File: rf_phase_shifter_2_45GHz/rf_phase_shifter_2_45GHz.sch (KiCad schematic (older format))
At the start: 12 parts, among them J1 CON-SMA-EDGE-S, J2 CON-SMA-EDGE-S, J3 CON-SMA-EDGE-S

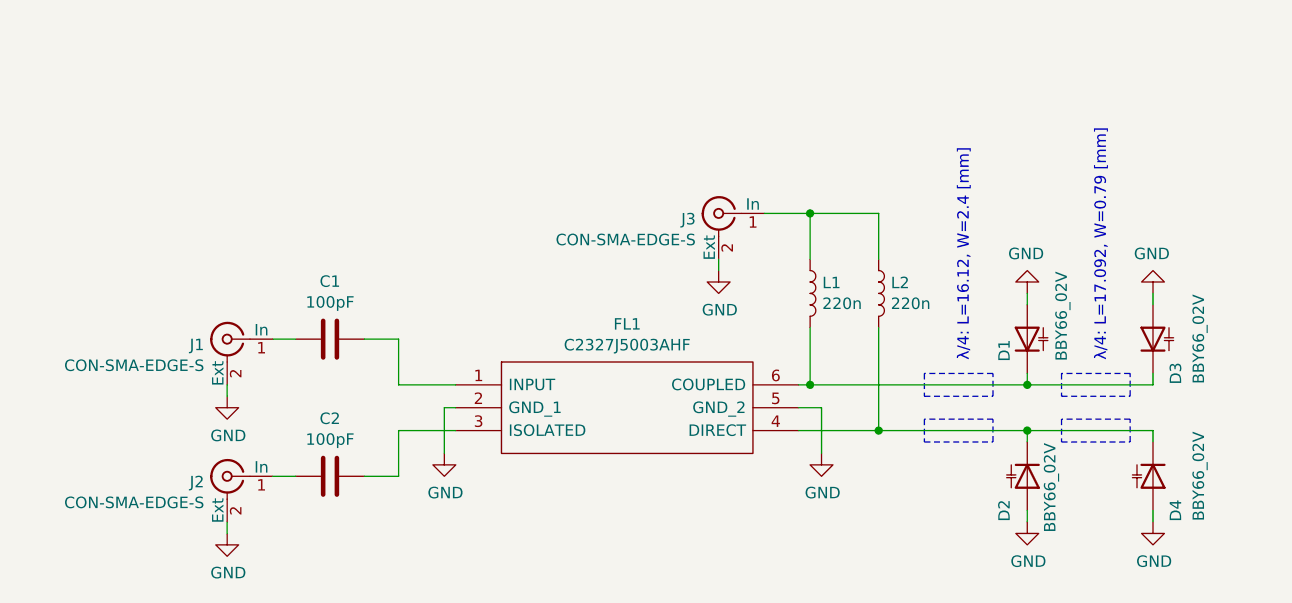
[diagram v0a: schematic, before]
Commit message: finished pcb layouts
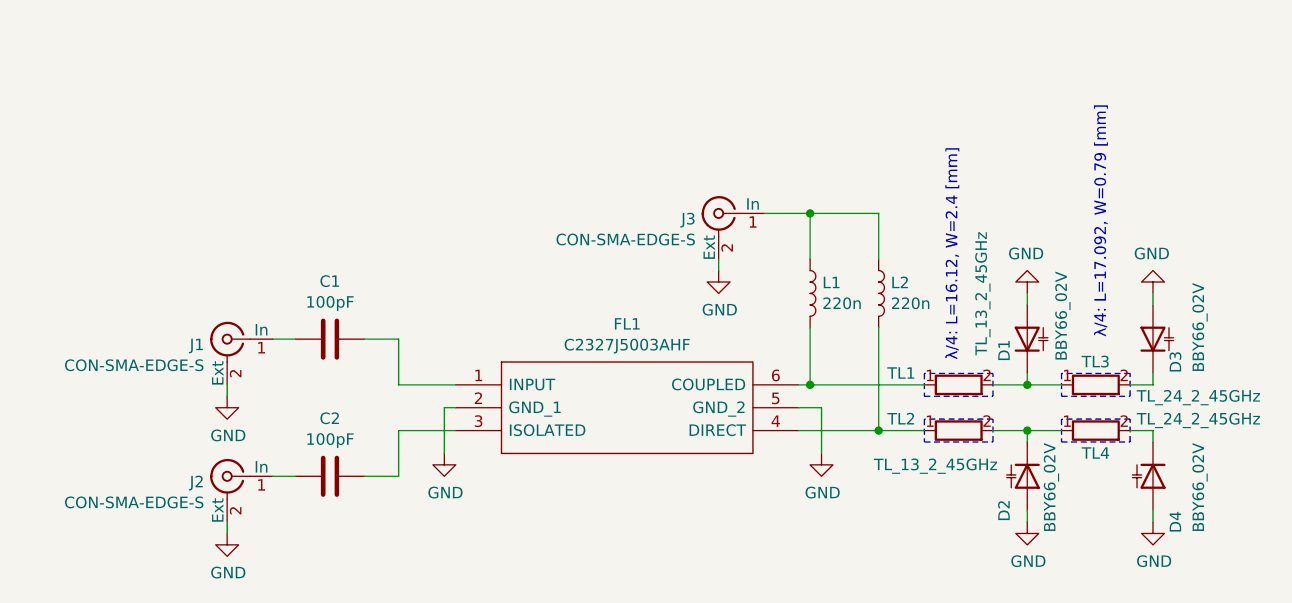
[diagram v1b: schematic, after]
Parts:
- added TL1, TL2: TL_13_2_45GHz, analog_rf_phase_shifter_module:TL_13_2_45GHz, symbol analog_rf_phase_shifter_module:TL_13_2_45GHz
- added TL3, TL4: TL_24_2_45GHz, analog_rf_phase_shifter_module:TL_24_2_45GHz, symbol analog_rf_phase_shifter_module:TL_24_2_45GHz
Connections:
- net at FL1.6 (COUPLED), L1.2: now also TL1.1; no longer D1.1 (K), D3.1 (K)
- net at FL1.4 (DIRECT), L2.2: now also TL2.1; no longer D2.1 (K), D4.1 (K)
- new net: D1.1 (K), TL1.2, TL3.1
- new net: D2.1 (K), TL2.2, TL4.1
- new net: D3.1 (K), TL3.2
- new net: D4.1 (K), TL4.2
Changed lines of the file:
@@
 U 1 1 60376509
 P 5600 2550
-F 0 "D4" H 5750 2650 50  0000 C CNN
-F 1 "BBY66_02V" H 5600 2750 50  0000 C CNN
+F 0 "D4" H 5800 2650 50  0000 C CNN
+F 1 "BBY66_02V" H 5650 2750 50  0000 C CNN
 F 2 "Diode_SMD:D_SOD-523" H 5600 2550 50  0001 C CNN
 F 3 "~" H 5600 2550 50  0001 C CNN
@@
 U 1 1 60375EF1
 P 5600 1950
-F 0 "D3" H 5450 1850 50  0000 C CNN
-F 1 "BBY66_02V" H 5600 1750 50  0000 C CNN
+F 0 "D3" H 5500 1850 50  0000 C CNN
+F 1 "BBY66_02V" H 5650 1750 50  0000 C CNN
 F 2 "Diode_SMD:D_SOD-523" H 5600 1950 50  0001 C CNN
 F 3 "~" H 5600 1950 50  0001 C CNN
@@
 $EndComp
 Wire Wire Line
-	5050 2150 5600 2150
-Wire Wire Line
-	5050 2350 5600 2350
-Wire Wire Line
-	4400 2350 5050 2350
+	5050 2150 5200 2150
+Wire Wire Line
+	5050 2350 5200 2350
+Wire Wire Line
+	4400 2350 4600 2350
 Connection ~ 5050 2150
 Connection ~ 4100 2150
 Wire Wire Line
-	4100 2150 5050 2150
-Text Notes 4800 2050 1    50   ~ 0
+	4100 2150 4600 2150
+Text Notes 4750 2050 1    50   ~ 0
 λ/4: L=16.12, W=2.4 [mm]
 Wire Notes Line
@@
 Wire Wire Line
 	2300 2350 2300 2550
-Text Notes 5400 2050 1    50   ~ 0
+Text Notes 5400 1950 1    50   ~ 0
 λ/4: L=17.092, W=0.79 [mm]
 $Comp
@@
 	1    0    0    -1
 $EndComp
+$Comp
+L analog_rf_phase_shifter_module:TL_13_2_45GHz TL1
+U 1 1 61540646
+P 4750 2100
+F 0 "TL1" H 4500 2100 50  0000 C CNN
+F 1 "TL_13_2_45GHz" V 4850 2450 50  0000 C CNN
+F 2 "analog_rf_phase_shifter_module:TL_13_2_45GHz" H 4500 2250 50  0001 C CNN
+F 3 "" H 4500 2250 50  0001 C CNN
+	1    4750 2100
+	1    0    0    -1
+$EndComp
+Wire Wire Line
+	4900 2150 5050 2150
+$Comp
+L analog_rf_phase_shifter_module:TL_13_2_45GHz TL2
+U 1 1 61540E40
+P 4750 2300
+F 0 "TL2" H 4500 2300 50  0000 C CNN
+F 1 "TL_13_2_45GHz" H 4650 2100 50  0000 C CNN
+F 2 "analog_rf_phase_shifter_module:TL_13_2_45GHz" H 4500 2450 50  0001 C CNN
+F 3 "" H 4500 2450 50  0001 C CNN
+	1    4750 2300
+	1    0    0    -1
+$EndComp
+Wire Wire Line
+	4900 2350 5050 2350
+$Comp
+L analog_rf_phase_shifter_module:TL_24_2_45GHz TL3
+U 1 1 61541F99
+P 5350 2100
+F 0 "TL3" H 5350 2150 50  0000 C CNN
+F 1 "TL_24_2_45GHz" H 5800 2000 50  0000 C CNN
+F 2 "analog_rf_phase_shifter_module:TL_24_2_45GHz" H 5100 2250 50  0001 C CNN
+F 3 "" H 5100 2250 50  0001 C CNN
+	1    5350 2100
+	1    0    0    -1
+$EndComp
+Wire Wire Line
+	5500 2150 5600 2150
+$Comp
+L analog_rf_phase_shifter_module:TL_24_2_45GHz TL4
+U 1 1 615424E1
+P 5350 2300
+F 0 "TL4" H 5350 2150 50  0000 C CNN
+F 1 "TL_24_2_45GHz" H 5800 2300 50  0000 C CNN
+F 2 "analog_rf_phase_shifter_module:TL_24_2_45GHz" H 5100 2450 50  0001 C CNN
+F 3 "" H 5100 2450 50  0001 C CNN
+	1    5350 2300
+	1    0    0    -1
+$EndComp
+Wire Wire Line
+	5500 2350 5600 2350
 $EndSCHEMATC
